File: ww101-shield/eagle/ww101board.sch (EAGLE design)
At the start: 53 parts, among them U1 ARDUINO_SHIELDNOHOLESORLABELS

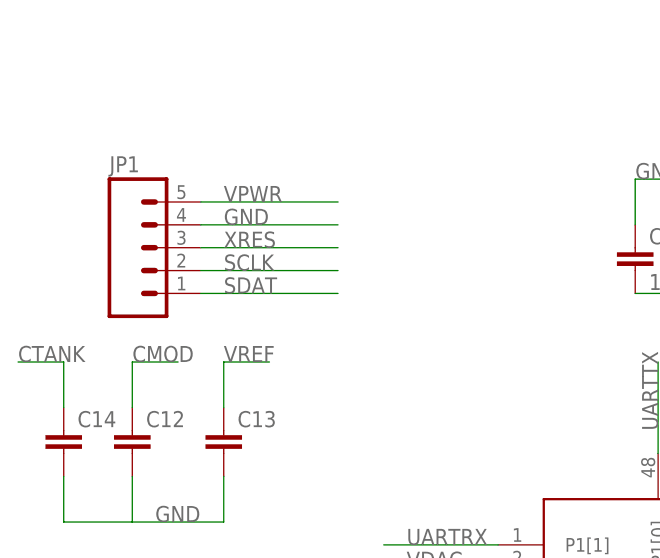
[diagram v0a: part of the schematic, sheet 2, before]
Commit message: routing complete
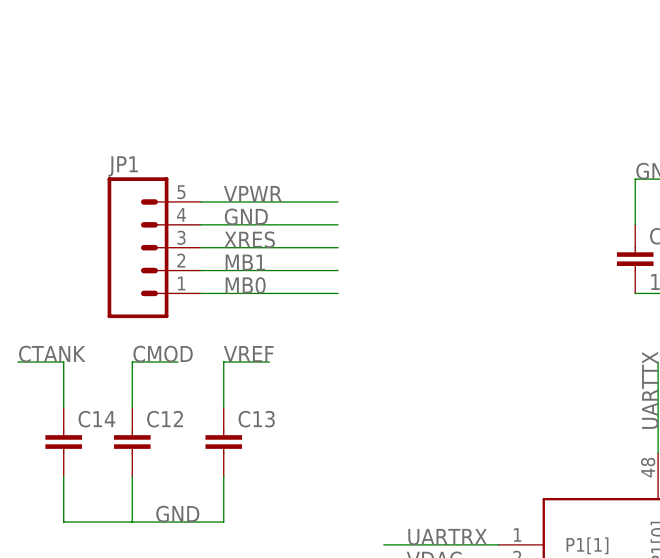
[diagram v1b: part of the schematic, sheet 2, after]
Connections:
- removed net SCLK: JP1.2
- removed net SDAT: JP1.1
- net MB0: now also JP1.1
- net MB1: now also JP1.2
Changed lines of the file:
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@@
 <label x="76.2" y="58.42" size="1.778" layer="95"/>
+</segment>
+<segment>
+<pinref part="JP1" gate="G$1" pin="1"/>
+<wire x1="-25.4" y1="106.68" x2="-10.16" y2="106.68" width="0.1524" layer="91"/>
+<label x="-22.86" y="106.68" size="1.778" layer="95"/>
 </segment>
 </net>
@@
 <wire x1="71.12" y1="60.96" x2="83.82" y2="60.96" width="0.1524" layer="91"/>
 <label x="76.2" y="60.96" size="1.778" layer="95"/>
+</segment>
+<segment>
+<pinref part="JP1" gate="G$1" pin="2"/>
+<wire x1="-25.4" y1="109.22" x2="-10.16" y2="109.22" width="0.1524" layer="91"/>
+<label x="-22.86" y="109.22" size="1.778" layer="95"/>
 </segment>
 </net>
@@
 </segment>
 </net>
-<net name="SDAT" class="0">
-<segment>
-<pinref part="JP1" gate="G$1" pin="1"/>
-<wire x1="-25.4" y1="106.68" x2="-10.16" y2="106.68" width="0.1524" layer="91"/>
-<label x="-22.86" y="106.68" size="1.778" layer="95"/>
-</segment>
-</net>
-<net name="SCLK" class="0">
-<segment>
-<pinref part="JP1" gate="G$1" pin="2"/>
-<wire x1="-25.4" y1="109.22" x2="-10.16" y2="109.22" width="0.1524" layer="91"/>
-<label x="-22.86" y="109.22" size="1.778" layer="95"/>
-</segment>
-</net>
